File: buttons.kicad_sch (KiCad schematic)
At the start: 91 parts, among them SW1 TC002-N11AS2XT-RGB, SW10 TC002-N11AS2XT-RGB, SW11 TC002-N11AS2XT-RGB, SW12 TC002-N11AS2XT-RGB, SW13 TC002-N11AS2XT-RGB, SW2 TC002-N11AS2XT-RGB, SW3 TC002-N11AS2XT-RGB, SW4 TC002-N11AS2XT-RGB, SW5 TC002-N11AS2XT-RGB, SW6 TC002-N11AS2XT-RGB, SW7 TC002-N11AS2XT-RGB, SW8 TC002-N11AS2XT-RGB, SW9 TC002-N11AS2XT-RGB, U17 WS2811F, U18 WS2811F, U19 WS2811F, U20 WS2811F, U21 WS2811F, U22 WS2811F, U23 WS2811F, U24 WS2811F, U25 WS2811F, U26 WS2811F, U27 WS2811F, U28 WS2811F, U29 WS2811F

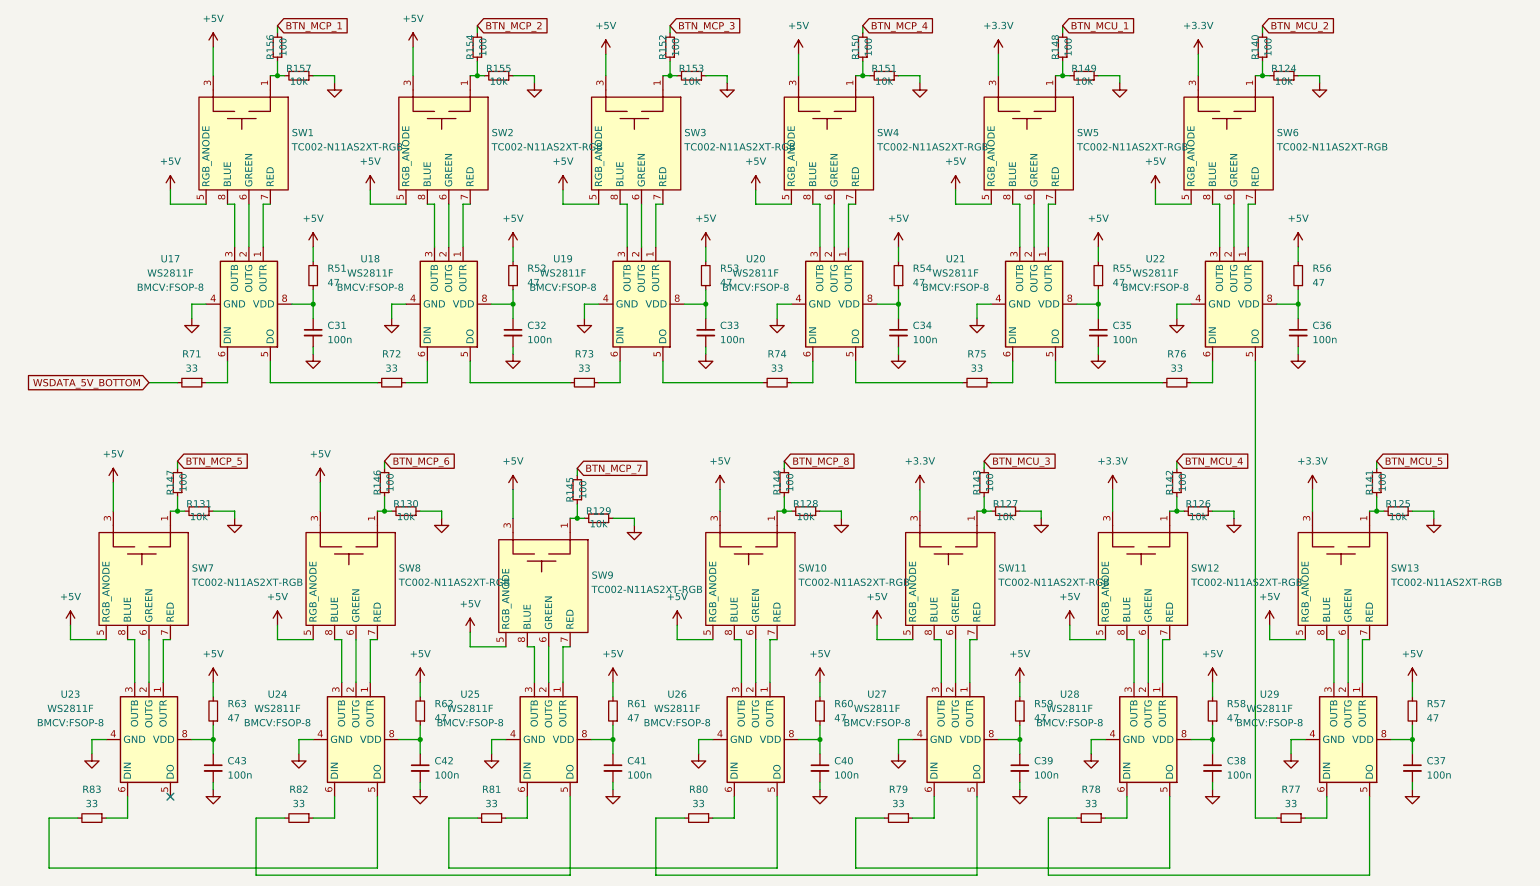
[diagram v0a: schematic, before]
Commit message: alpha
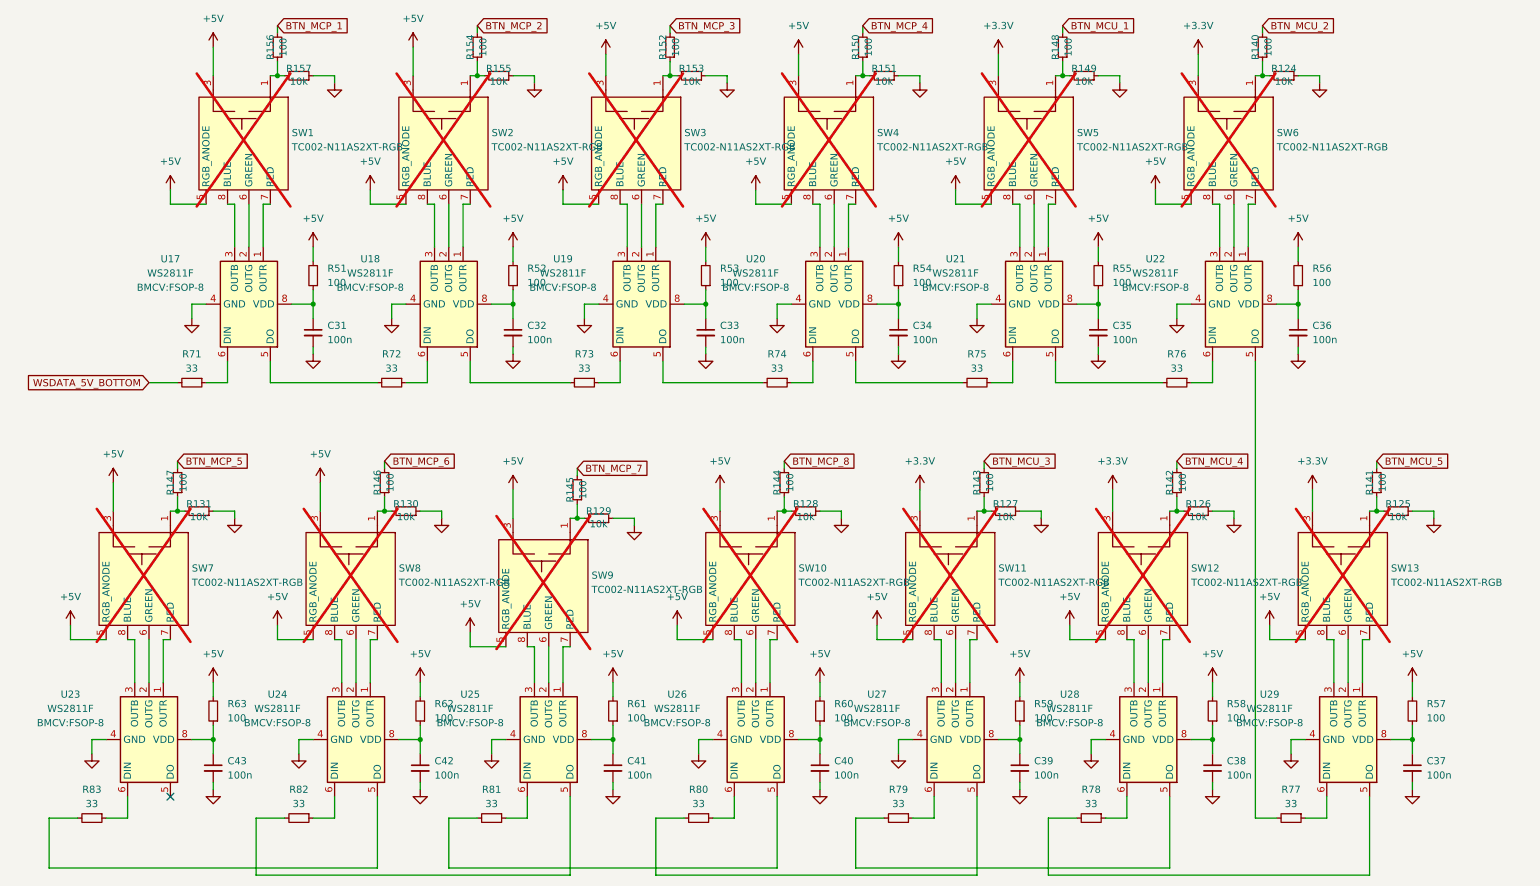
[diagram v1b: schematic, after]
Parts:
- C31, C32, C33, C34, C35, C36, C37, C38, C39, C40, C41, C42, C43: LCSC Part # (none) -> C307331
- R124, R125, R126, R127, R128, R129, R130, R131, R149, R151, R153, R155, R157: LCSC Part # (none) -> C25744
- R140, R141, R142, R143, R144, R145, R146, R147, R148, R150, R152, R154, R156: LCSC Part # (none) -> C25076
- R51, R52, R53, R54, R55, R56, R57, R58, R59, R60, R61, R62, R63: value 47 -> 100; LCSC Part # (none) -> C25076
- R71, R72, R73, R74, R75, R76, R77, R78, R79, R80, R81, R82, R83: LCSC Part # (none) -> C25105
- SW1, SW10, SW11, SW12, SW13, SW2, SW3, SW4, SW5, SW6, SW7, SW8, SW9: now not fitted
- U17, U18, U19, U20, U21, U22, U23, U24, U25, U26, U27, U28, U29: LCSC Part # (none) -> C5446692
